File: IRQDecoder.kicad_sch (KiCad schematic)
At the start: 6 parts, among them U17 74HC138, U18 74HC148, U20 74HC373, U4 74HC32

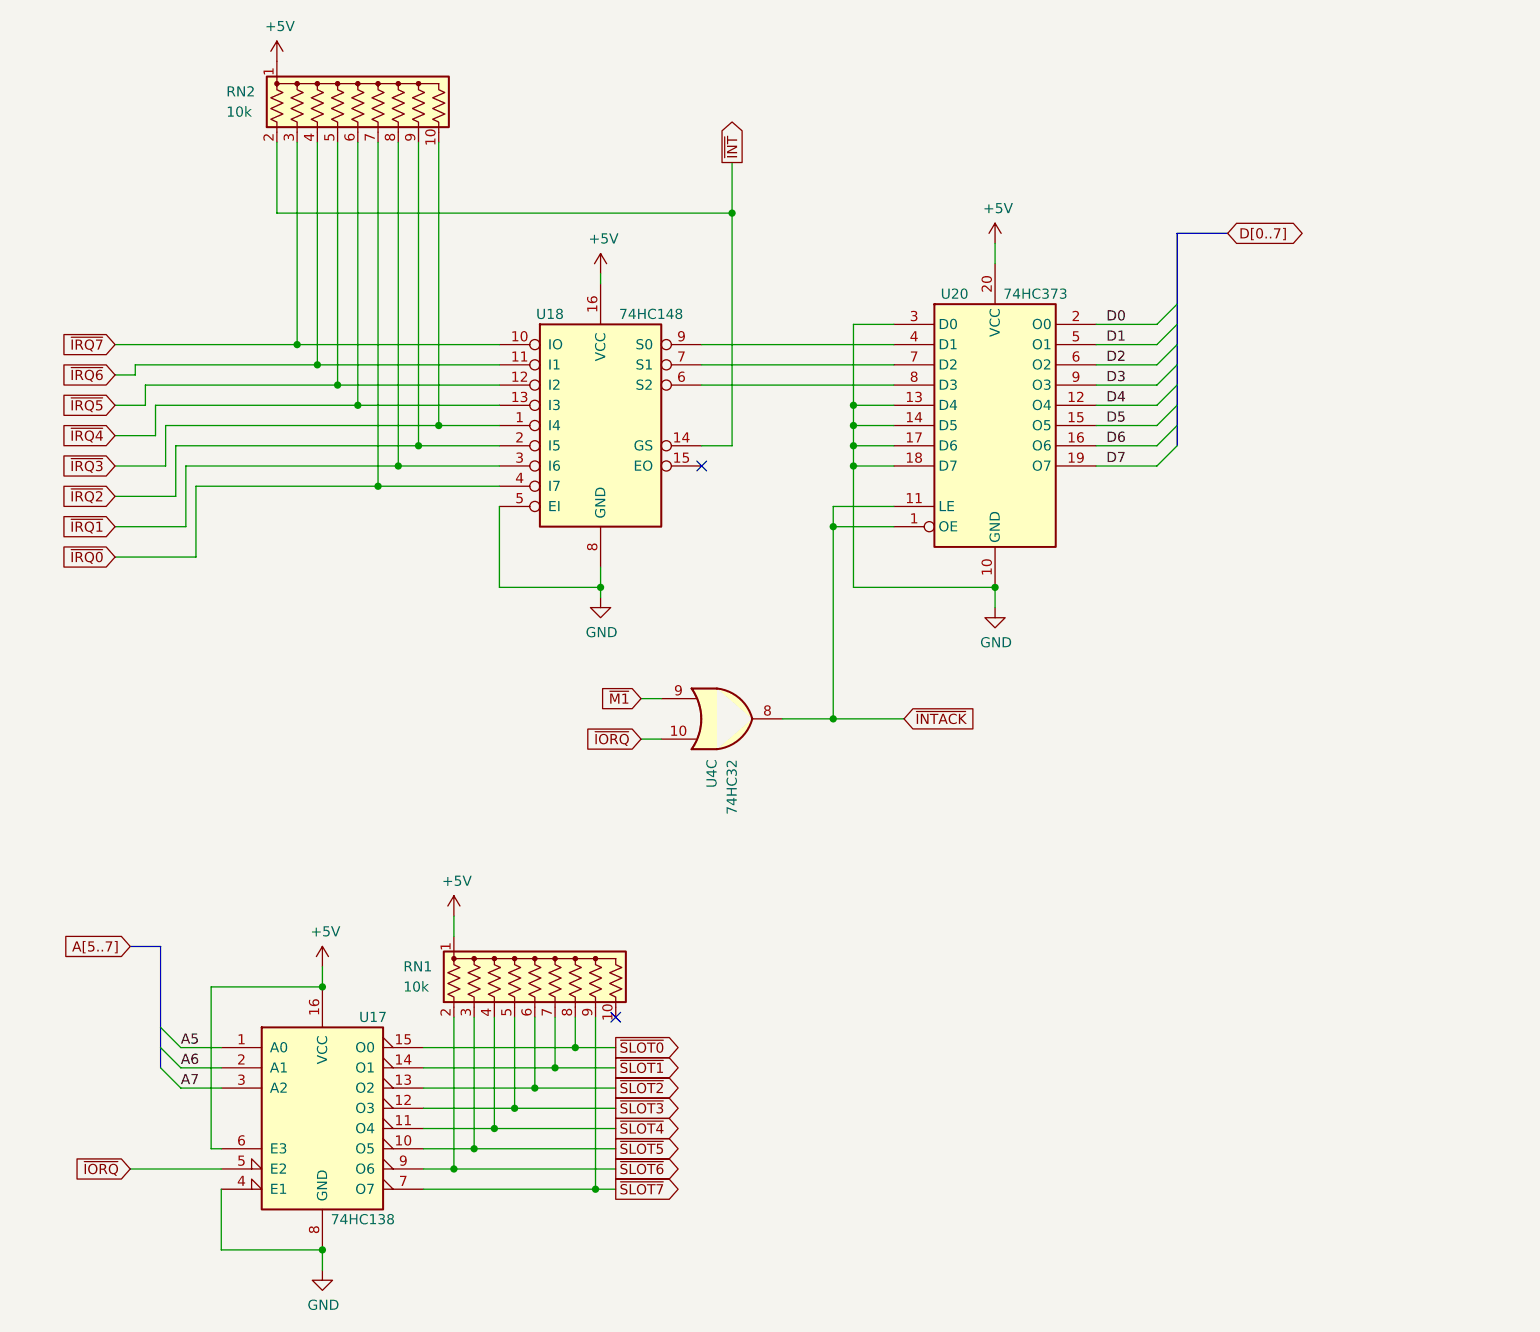
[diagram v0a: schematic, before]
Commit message: Schematic cleanup
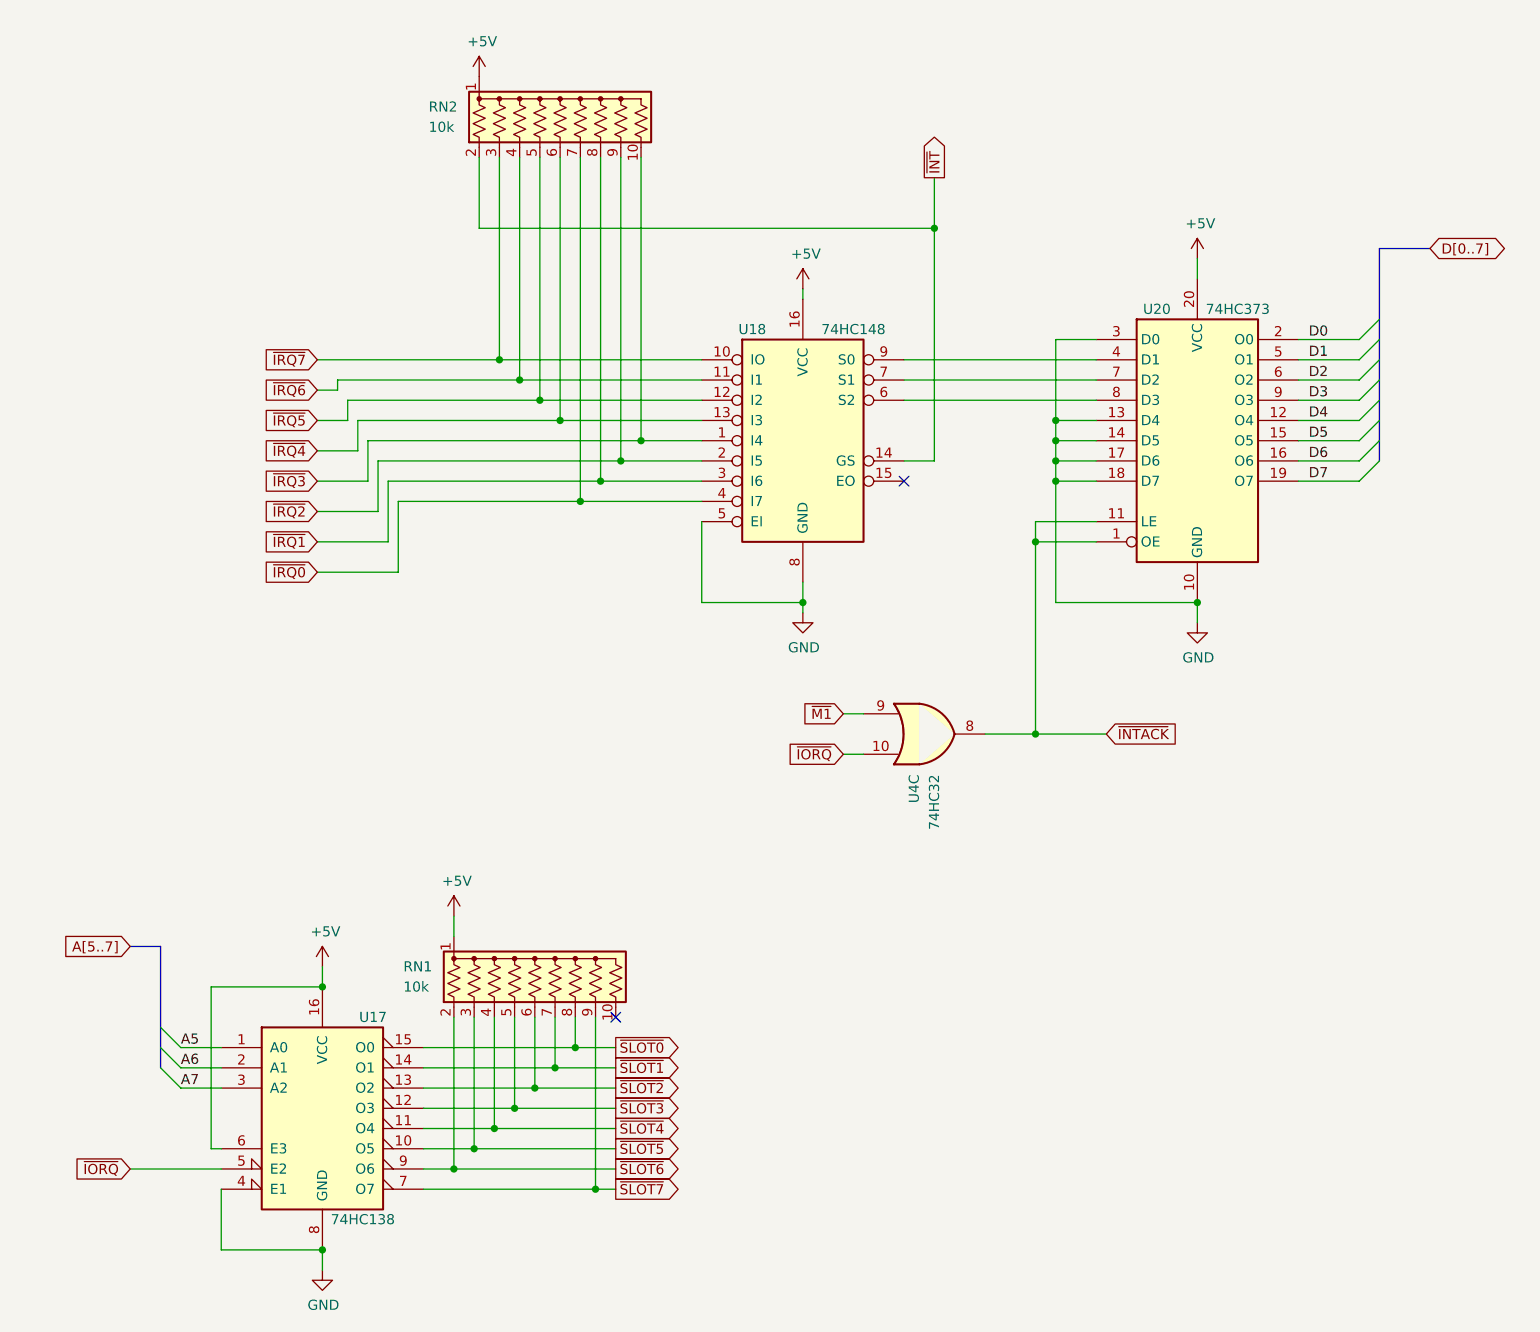
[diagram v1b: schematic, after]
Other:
- moved on the sheet: RN2, U18, U20, U4C
